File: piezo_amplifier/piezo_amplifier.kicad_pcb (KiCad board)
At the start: 2 copper layers, 40 x 23.5 mm, 23 parts, among them J1 Conn_01x02_Female, J2 Conn_01x02_Female, J3 Conn_01x02_Female, J4 Conn_01x02_Female, U1 LMV324, U2 TLV76033DBZT

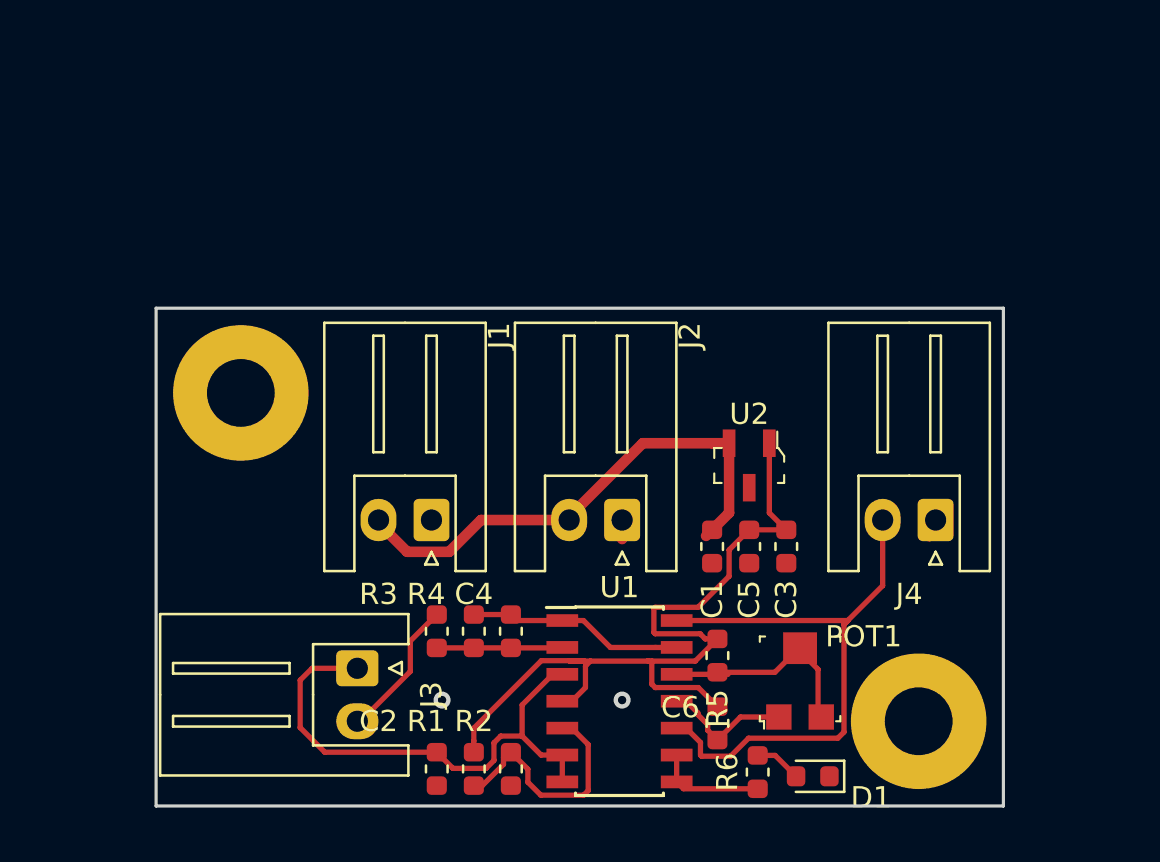
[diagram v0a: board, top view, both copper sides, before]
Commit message: PCB and schematics files finished, ready for release.
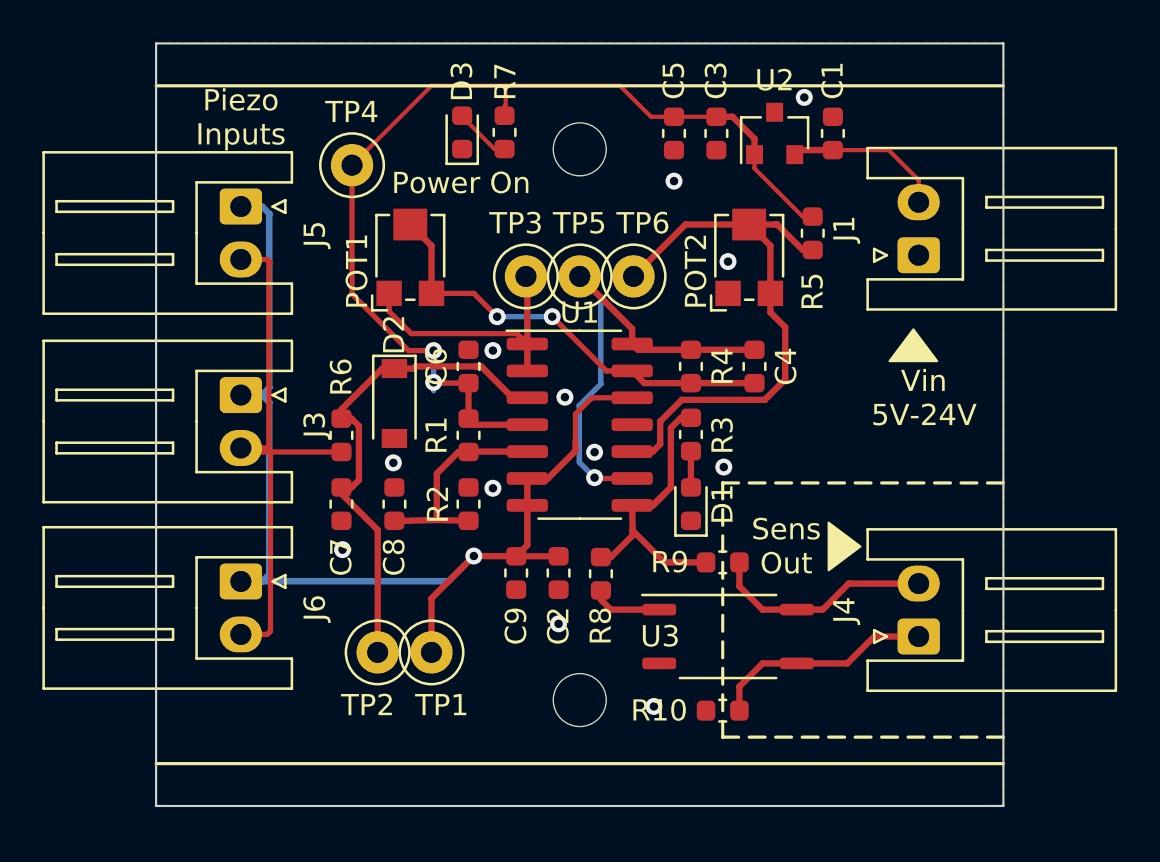
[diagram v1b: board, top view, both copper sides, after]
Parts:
- removed J2: Conn_01x02_Female, Connector_JST:JST_XH_S02B-XH-A_1x02_P2.50mm_Horizontal
- removed the REF** at (141.0, 91.0)
- removed the REF** at (109.0, 75.5)
- added C7: 22nF, Capacitor_SMD:C_0603_1608Metric, F.Cu at (113.8, 80.8)
- added C8: 22nF, Capacitor_SMD:C_0603_1608Metric, F.Cu at (116.2, 80.8)
- added C9: 1uF, Capacitor_SMD:C_0603_1608Metric, F.Cu at (122.0, 84.0)
- added D2: TVS_5V, Diode_SMD:D_SOD-123, F.Cu at (116.2, 76.0)
- added D3: LED, LED_SMD:LED_0603_1608Metric, F.Cu at (119.5, 63.2)
- added J5: Conn_01x02_Female, Connector_JST:JST_XH_S2B-XH-A_1x02_P2.50mm_Horizontal, F.Cu at (109.0, 66.7)
- added J6: Conn_01x02_Female, Connector_JST:JST_XH_S2B-XH-A_1x02_P2.50mm_Horizontal, F.Cu at (109.0, 84.4)
- added POT2: TC33X-2-103E, Potentiometer_SMD:Potentiometer_Bourns_TC33X_Vertical, F.Cu at (133.0, 69.0)
- added R10: 0R, Resistor_SMD:R_0603_1608Metric, F.Cu at (131.8, 90.5)
- added R7: 330, Resistor_SMD:R_0603_1608Metric, F.Cu at (121.5, 63.2)
- added R8: 330R, Resistor_SMD:R_0603_1608Metric, F.Cu at (126.0, 84.0)
- added R9: 0R, Resistor_SMD:R_0603_1608Metric, F.Cu at (131.8, 83.5)
- added REF**: MountingHole_2.5mm, MountingHole:MountingHole_2.5mm, F.Cu at (125.0, 64.0)
- added REF**: MountingHole_2.5mm, MountingHole:MountingHole_2.5mm, F.Cu at (125.0, 90.0)
- added TP1: TestPoint, TestPoint:TestPoint_Loop_D1.80mm_Drill1.0mm_Beaded, F.Cu at (118.0, 87.8)
- added TP2: TestPoint, TestPoint:TestPoint_Loop_D1.80mm_Drill1.0mm_Beaded, F.Cu at (115.5, 87.8)
- added TP3: TestPoint, TestPoint:TestPoint_Loop_D1.80mm_Drill1.0mm_Beaded, F.Cu at (122.5, 70.0)
- added TP4: TestPoint, TestPoint:TestPoint_Loop_D1.80mm_Drill1.0mm_Beaded, F.Cu at (114.2, 64.8)
- added TP5: TestPoint, TestPoint:TestPoint_Loop_D1.80mm_Drill1.0mm_Beaded, F.Cu at (125.0, 70.0)
- added TP6: TestPoint, TestPoint:TestPoint_Loop_D1.80mm_Drill1.0mm_Beaded, F.Cu at (127.5, 70.0)
- added U3: TLP185, Package_SO:SOIC-4_4.55x3.7mm_P2.54mm, F.Cu at (132.0, 87.0)
- J1, J3, J4: footprint Connector_JST:JST_XH_S02B-XH-A_1x02_P2.50mm_Horizontal -> Connector_JST:JST_XH_S2B-XH-A_1x02_P2.50mm_Horizontal
- POT1: value TC33X-2-103E -> 10K; footprint digikey-footprints:Trimpot_3.8mmx3.6mm_TC33X-2-103E -> Potentiometer_SMD:Potentiometer_Bourns_TC33X_Vertical
- R3: value 10K -> 330
- R4: value 10K -> 20K
- R6: value 100 -> 10K
- U2: footprint digikey-footprints:SOT-23-3 -> Package_TO_SOT_SMD:SOT-23
- moved POT1 27.2 mm to (117.0, 69.0), turned to 90 degrees
- moved J1 26.2 mm to (141.0, 69.0), turned to 90 degrees
- moved R6 25.3 mm to (113.8, 77.5), turned to 270 degrees
- moved C6 20.5 mm to (119.8, 74.2), turned to 270 degrees
- moved R5 20.4 mm to (136.0, 68.0)
- moved C1 20.3 mm to (136.9, 63.2), turned to 270 degrees
- moved C5 19.8 mm to (129.4, 63.2)
- moved C3 19.8 mm to (131.4, 63.2)
- moved C4 17.0 mm to (133.2, 74.2)
- moved R4 16.2 mm to (130.2, 74.2)
- moved R1 15.8 mm to (119.8, 77.5)
- moved U2 15.7 mm to (134.2, 63.2), turned to 90 degrees
- moved R3 15.2 mm to (130.2, 77.5)
- moved D1 14.1 mm to (130.2, 80.8), turned to 90 degrees
- moved J3 14.0 mm to (109.0, 75.6)
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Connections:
- J4 pad 1: GND -> Net-(J4-Pad1)
- POT1 pad 1: GND -> Net-(POT1-Pad1)
- POT1 pad 2: Net-(POT1-Pad2) -> Net-(C4-Pad2)
- POT1 pad 3: Net-(POT1-Pad2) -> Net-(C4-Pad2)
- R3 pad 1: Net-(C4-Pad2) -> Net-(D1-Pad2)
- R3 pad 2: Net-(J3-Pad2) -> Net-(R3-Pad2)
- R5 pad 2: Net-(POT1-Pad2) -> Net-(POT2-Pad2)
- R6 pad 1: Net-(R6-Pad1) -> Net-(C7-Pad2)
- R6 pad 2: Net-(D1-Pad2) -> Net-(J3-Pad2)
- U1 pad 1: Net-(C4-Pad1) -> Net-(POT1-Pad1)
- U1 pad 10: /Probe_Out -> Net-(POT2-Pad2)
- U1 pad 12: Net-(POT1-Pad2) -> /Vref
- U1 pad 13: Net-(C4-Pad1) -> Net-(C4-Pad2)
- U1 pad 14: /Probe_Out -> Net-(C4-Pad1)
- U1 pad 2: Net-(C4-Pad2) -> Net-(POT1-Pad1)
- U1 pad 3: /Vref -> Net-(C7-Pad2)
- U1 pad 8: Net-(R6-Pad1) -> Net-(R3-Pad2)
- U1 pad 9: Net-(R6-Pad1) -> Net-(C4-Pad1)
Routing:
- net /Vref: track 25.5 -> 53.6 mm, vias 0 -> 1
- net Net-(POT2-Pad2): track 0.00 -> 27.8 mm
- net Net-(C7-Pad2): track 0.00 -> 23.8 mm
- net Net-(J3-Pad2): track 6.68 -> 26.7 mm
- net /Probe_Out: track 28.4 -> 10.6 mm
- net /Vin: track 24.3 -> 7.57 mm
- net Net-(C4-Pad2): track 5.93 -> 20.7 mm, vias 0 -> 2
- net Net-(R3-Pad2): track 0.00 -> 14.3 mm
- net Net-(POT1-Pad1): track 0.00 -> 12.5 mm
- net Net-(C4-Pad1): track 10.2 -> 22.5 mm, vias 0 -> 1
- net Net-(J4-Pad1): track 0.00 -> 10.6 mm
- net Net-(POT1-Pad2): track 10.1 -> 0.00 mm
- net +3V3: track 39.7 -> 46.9 mm, vias 0 -> 2
- net GND: track 6.54 -> 0.00 mm, vias 2 -> 12
- net Net-(R6-Pad1): track 5.47 -> 0.00 mm
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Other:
- board size 40 x 23.5 mm -> 40 x 36 mm
- board text added: "Piezo Inputs"
- board text added: "PiezoSaurus V2.0"
- board text added: "Power On"
- board text added: "Sens Out"
- board text added: "Vin 5V-24V"
- board text removed: "PiezoSaurus V1.0"
